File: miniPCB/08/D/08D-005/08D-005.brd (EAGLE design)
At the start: 42 parts

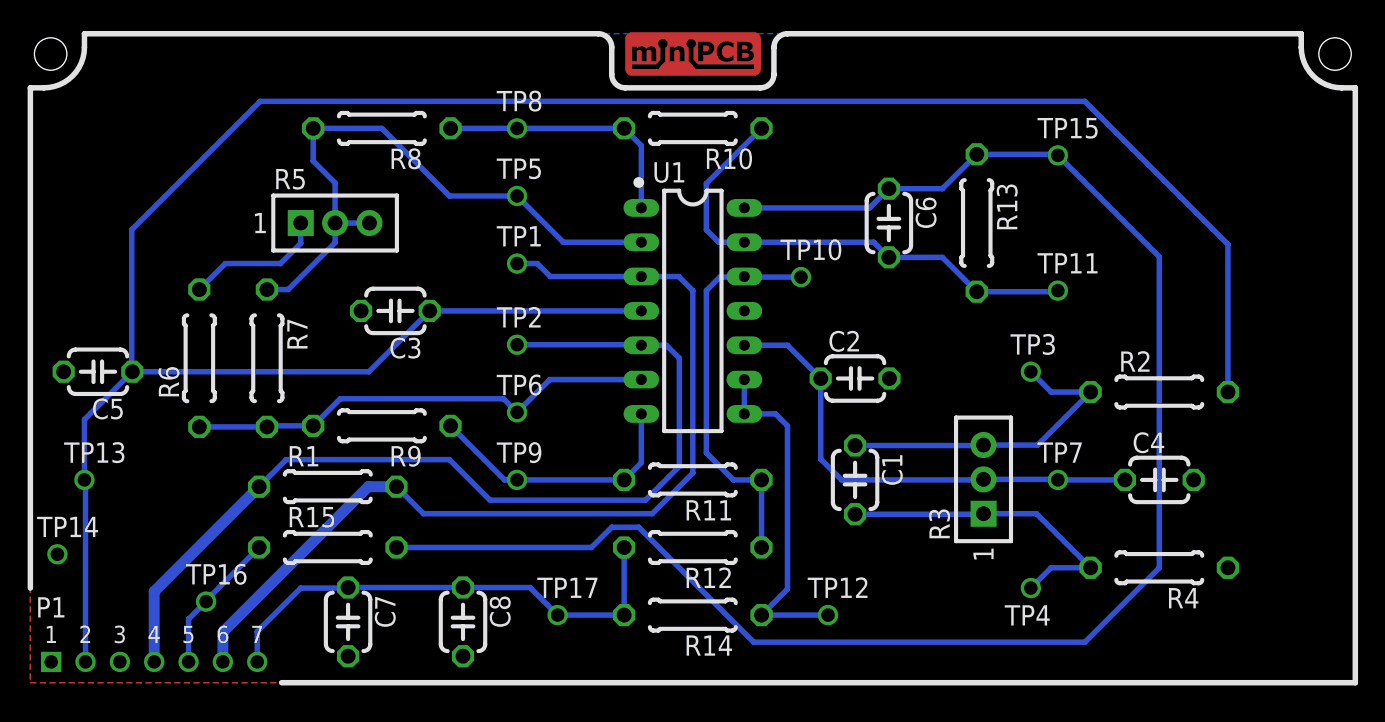
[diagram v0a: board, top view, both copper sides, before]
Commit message: Attempting to fix my Git merge error.
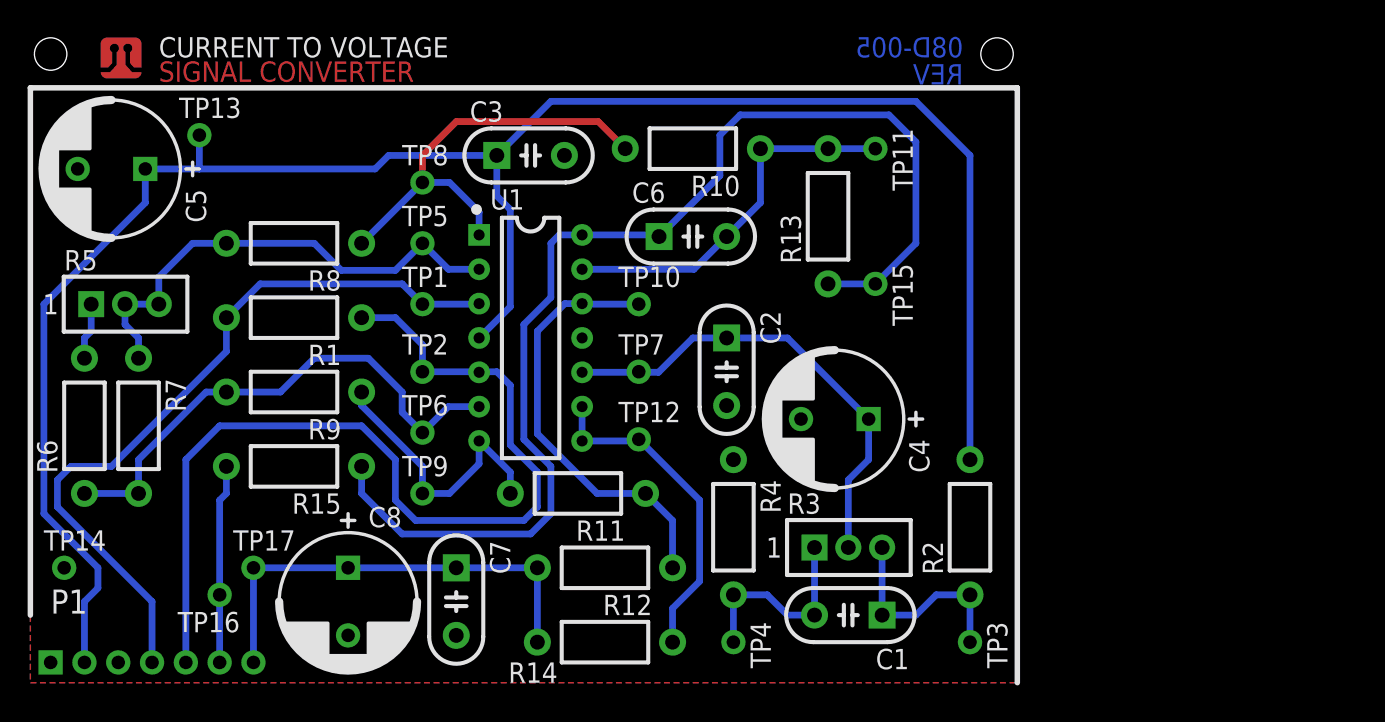
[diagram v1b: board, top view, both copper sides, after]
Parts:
- removed P1-: (no value), minipcb:MINIPCB_7P_50X100
- added P1: (no value), minipcb:PINS_1X7
- added PCB1: (no value), minipcb:MINIPCB_0P_50X75
- C4, C5, C8: device minipcb:C050-024X044 -> minipcb:C5MM
- moved TP7 32.0 mm to (46.0, 24.0)
- moved R4 31.6 mm to (53.0, 12.5), turned to 270 degrees
- moved TP13 26.9 mm to (13.5, 41.5)
- moved C4 24.4 mm to (60.5, 20.5), turned to 180 degrees
- moved TP17 22.8 mm to (17.5, 9.50)
- moved TP4 22.4 mm to (53.0, 4.00), turned to 270 degrees
- moved TP3 20.5 mm to (70.5, 4.00), turned to 270 degrees
- moved TP12 19.1 mm to (46.0, 19.0)
- moved R2 17.2 mm to (70.5, 12.5), turned to 90 degrees
- moved TP11 17.1 mm to (63.5, 40.5), turned to 270 degrees
- moved R5 16.6 mm to (5.50, 29.0)
- moved TP15 16.5 mm to (63.5, 30.5), turned to 270 degrees
- moved C3 15.2 mm to (38.0, 40.0), turned to 0 degrees
- moved C5 15.0 mm to (7.00, 39.0)
- moved C6 14.5 mm to (50.0, 34.0), turned to 0 degrees
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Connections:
- net BIAS: now also C4.+; no longer C4.1
- net GND: now also C4.-, C5.-, C8.-, P1.1; no longer C4.2, C5.2, C8.2, P1-.1
- net N$11: now also P1.6, R15.2; no longer P1-.5, R15.1
- net N$2: now also C8.+, P1.7; no longer C8.1, P1-.7
- net N$3: now also P1.5; no longer P1-.4
- net N$4: now also P1.4; no longer P1-.6
- net NC: now also P1.3; no longer P1-.3
- net OUT: now also R15.1; no longer R15.2
- net V+: now also C5.+, P1.2; no longer C5.1, P1-.2
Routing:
- net OUT: track 121.3 -> 88.4 mm
- net V+: track 173.4 -> 146.3 mm
- net N$4: track 70.8 -> 55.7 mm
- net N$7: track 19.2 -> 32.0 mm
- net N$5: track 45.9 -> 36.1 mm
- net VFB: track 37.1 -> 27.7 mm
- net POT.1: track 24.1 -> 15.1 mm
- net POT.3: track 24.1 -> 15.6 mm
- net N$10: track 10.4 -> 4.21 mm
- net N$11: track 10.6 -> 14.7 mm
- net N$6: track 35.0 -> 38.7 mm
- net N$2: track 36.6 -> 33.5 mm
- net N$1: track 29.4 -> 32.1 mm
- net N$9: track 25.8 -> 24.5 mm
- net N$8: track 19.9 -> 21.0 mm
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
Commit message: Attempting to fix my Git merge error.
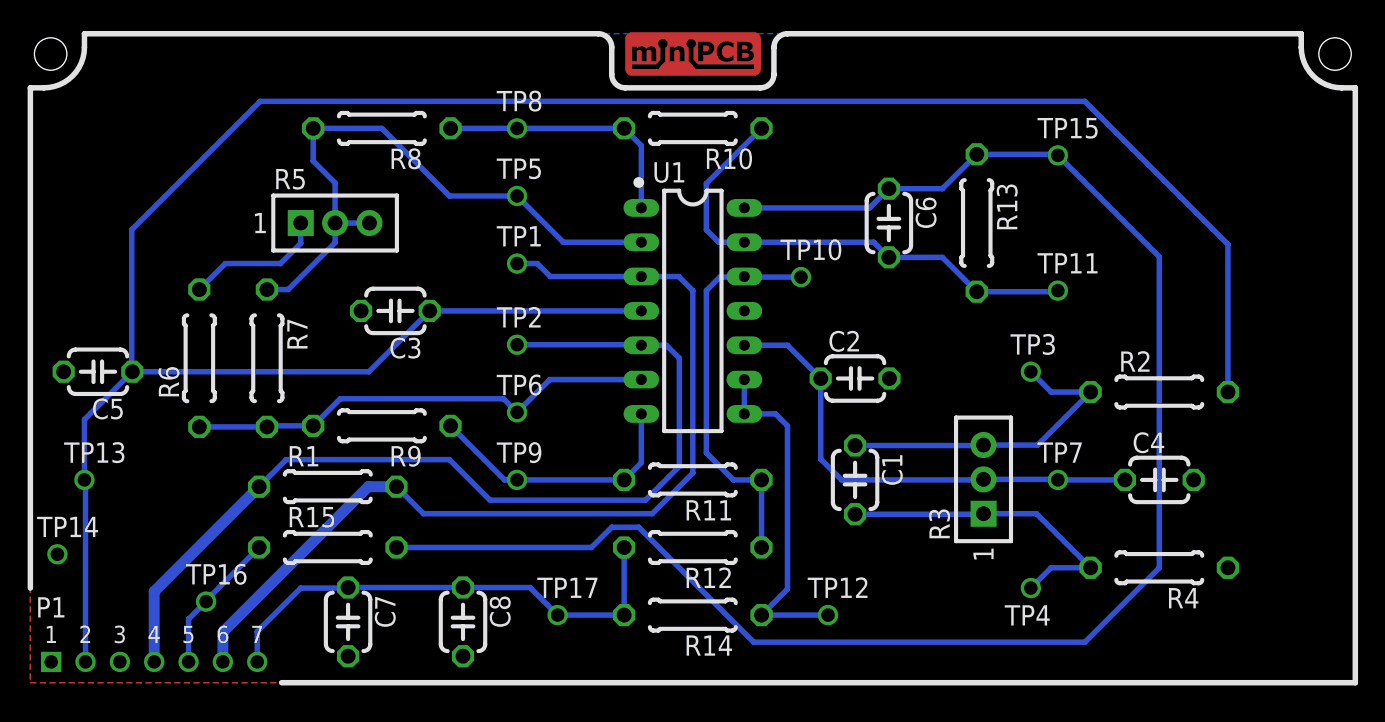
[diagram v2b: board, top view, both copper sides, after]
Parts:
- removed P1: (no value), minipcb:PINS_1X7
- removed PCB1: (no value), minipcb:MINIPCB_0P_50X75
- added P1-: (no value), minipcb:MINIPCB_7P_50X100
- C4, C5, C8: device minipcb:C5MM -> minipcb:C050-024X044
- moved TP7 32.0 mm to (77.0, 16.0)
- moved R4 31.6 mm to (84.5, 9.50), turned to 180 degrees
- moved TP13 26.9 mm to (5.00, 16.0)
- moved C4 24.4 mm to (84.5, 16.0), turned to 0 degrees
- moved TP17 22.8 mm to (40.0, 6.00)
- moved TP4 22.4 mm to (75.0, 8.00), turned to 180 degrees
- moved TP3 20.5 mm to (75.0, 24.0), turned to 0 degrees
- moved TP12 19.1 mm to (60.0, 6.00)
- moved R2 17.2 mm to (84.5, 22.5), turned to 0 degrees
- moved TP11 17.1 mm to (77.0, 30.0), turned to 0 degrees
- moved R5 16.6 mm to (21.0, 35.0)
- moved TP15 16.5 mm to (77.0, 40.0), turned to 0 degrees
- moved C3 15.2 mm to (28.0, 28.5), turned to 180 degrees
- moved C5 15.0 mm to (6.00, 24.0)
- moved C6 14.5 mm to (64.5, 35.0), turned to 270 degrees
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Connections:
- net BIAS: now also C4.1; no longer C4.+
- net GND: now also C4.2, C5.2, C8.2, P1-.1; no longer C4.-, C5.-, C8.-, P1.1
- net N$11: now also P1-.5, R15.1; no longer P1.6, R15.2
- net N$2: now also C8.1, P1-.7; no longer C8.+, P1.7
- net N$3: now also P1-.4; no longer P1.5
- net N$4: now also P1-.6; no longer P1.4
- net NC: now also P1-.3; no longer P1.3
- net OUT: now also R15.2; no longer R15.1
- net V+: now also C5.1, P1-.2; no longer C5.+, P1.2
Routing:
- net OUT: track 88.4 -> 121.3 mm
- net V+: track 146.3 -> 173.4 mm
- net N$4: track 55.7 -> 70.8 mm
- net N$7: track 32.0 -> 19.2 mm
- net N$5: track 36.1 -> 45.9 mm
- net VFB: track 27.7 -> 37.1 mm
- net POT.1: track 15.1 -> 24.1 mm
- net POT.3: track 15.6 -> 24.1 mm
- net N$10: track 4.21 -> 10.4 mm
- net N$11: track 14.7 -> 10.6 mm
- net N$6: track 38.7 -> 35.0 mm
- net N$2: track 33.5 -> 36.6 mm
- net N$1: track 32.1 -> 29.4 mm
- net N$9: track 24.5 -> 25.8 mm
- net N$8: track 21.0 -> 19.9 mm
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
